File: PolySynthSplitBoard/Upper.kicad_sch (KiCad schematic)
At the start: 3 parts, among them J801 A_UPPER, J802 B_UPPER, J803 C_UPPER

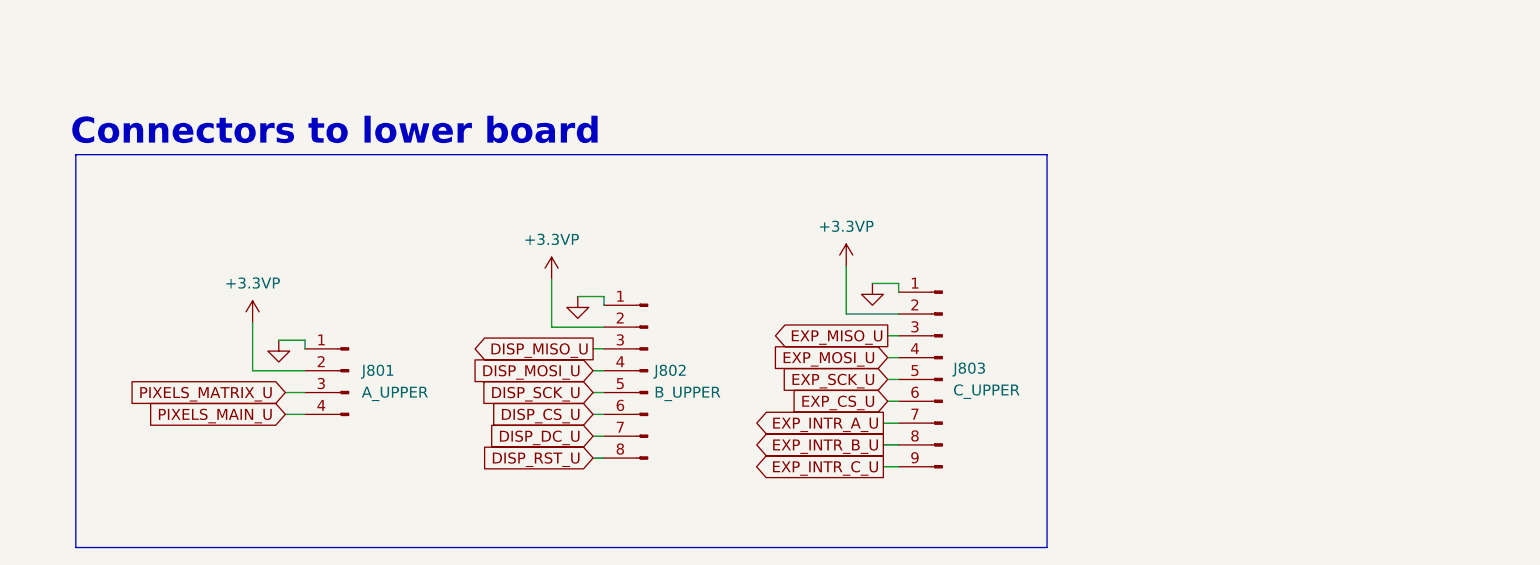
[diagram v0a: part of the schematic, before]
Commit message: lower board
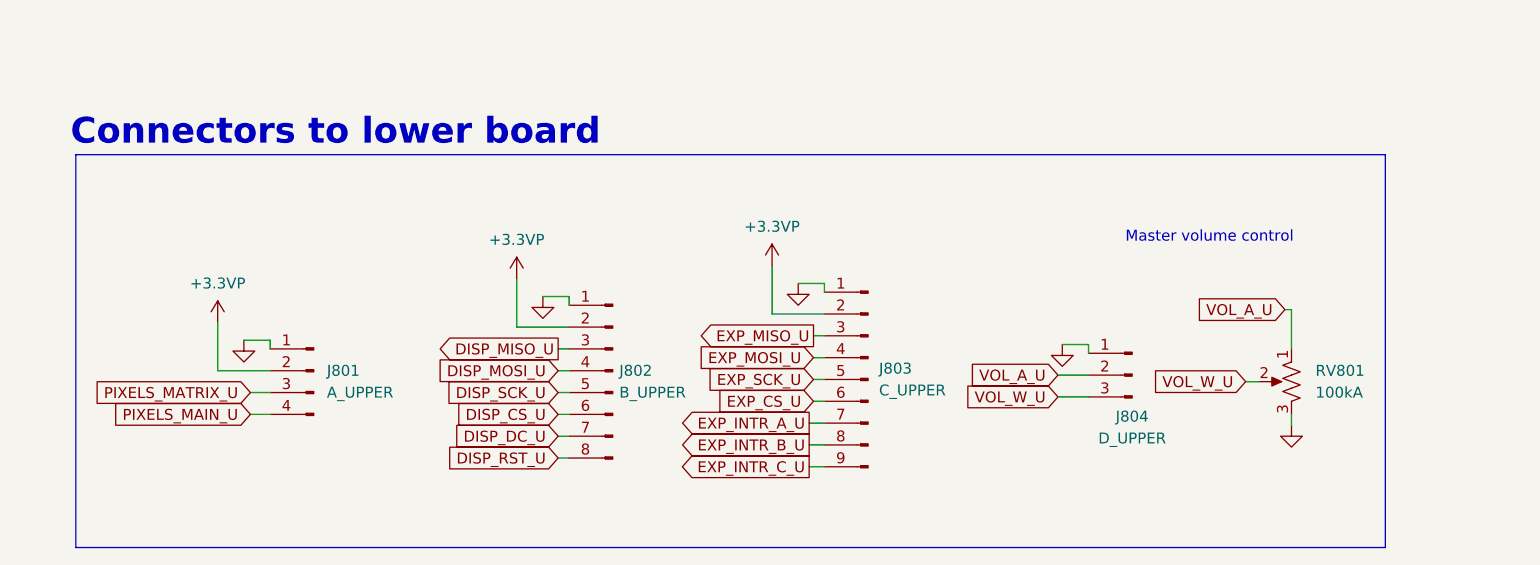
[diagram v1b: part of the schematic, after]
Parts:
- added J804: D_UPPER, Connector_PinSocket_2.54mm:PinSocket_1x03_P2.54mm_Vertical, symbol Connector:Conn_01x03_Pin
- added RV801: 100kA, Potentiometer_THT:Potentiometer_Bourns_PTV09A-1_Single_Vertical, symbol Device:R_Potentiometer_US
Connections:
- net GNDA: now also J804.1 (Pin_1), RV801.3
- new net VOL_A_U: J804.2 (Pin_2), RV801.1
- new net VOL_W_U: J804.3 (Pin_3), RV801.2
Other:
- note added: "Master volume control"
- moved on the sheet: J801, J802, J803
